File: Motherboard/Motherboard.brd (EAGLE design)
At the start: 87.5 x 150 mm, 11 parts

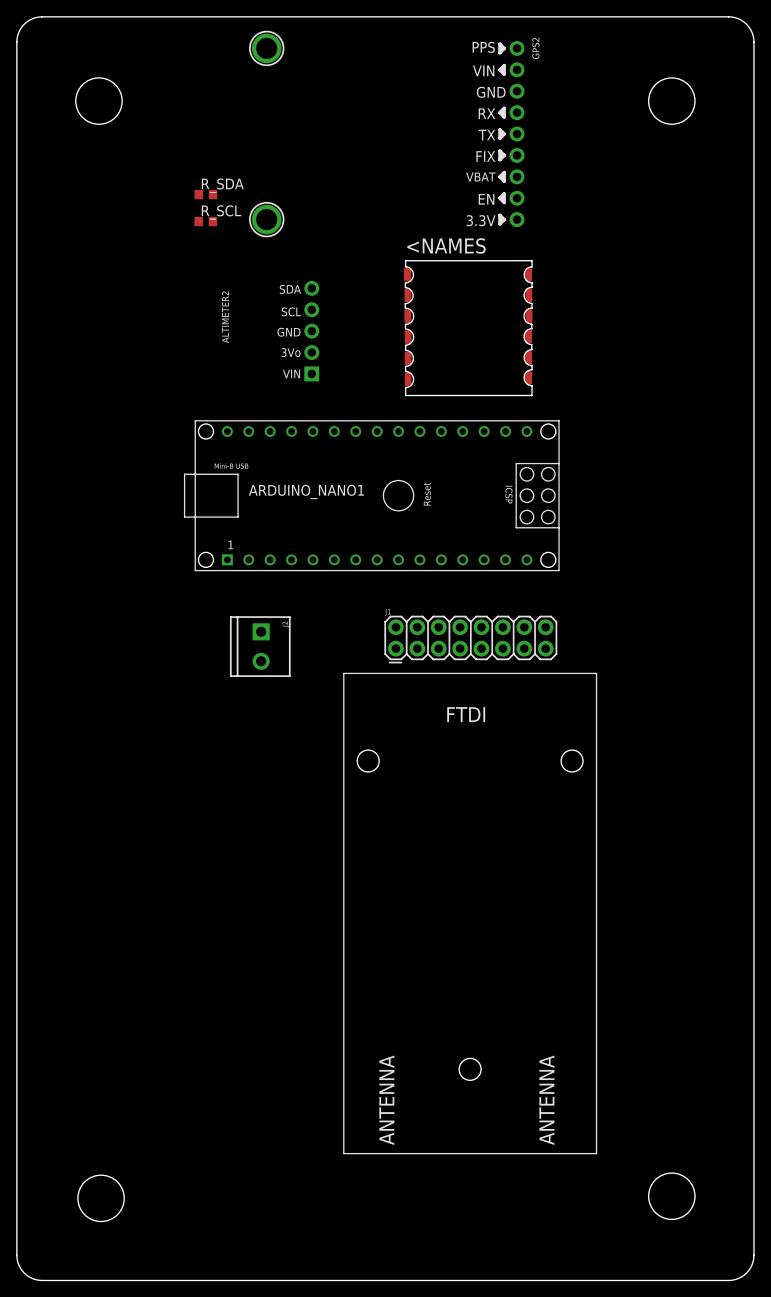
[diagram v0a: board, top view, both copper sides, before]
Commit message: refactor
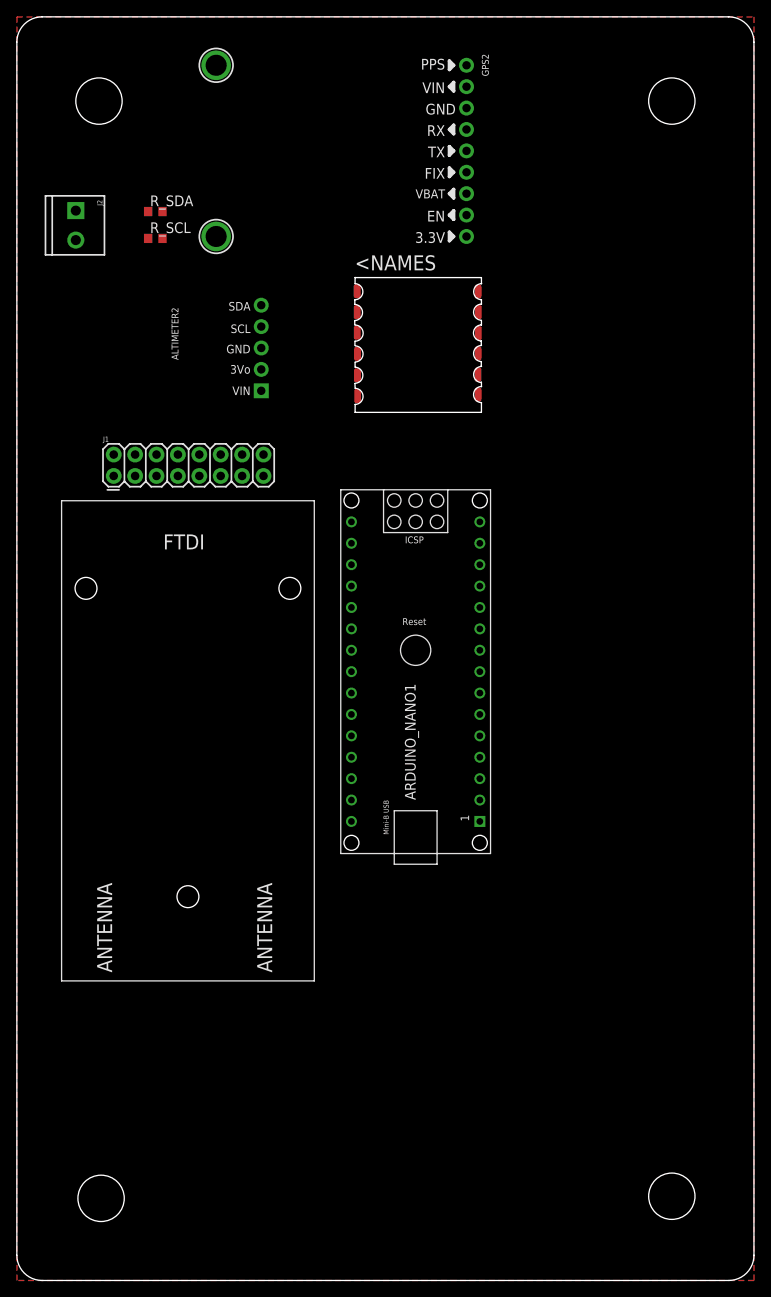
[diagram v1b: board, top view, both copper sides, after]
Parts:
- moved J2 54.6 mm to (7.00, 127.0)
- moved J1 39.3 mm to (11.5, 95.5)
- moved U$1 39.3 mm to (19.7, 64.0)
- moved ARDUINO_NANO1 18.5 mm to (47.3, 74.8), turned to 90 degrees
- moved GPS2 6.32 mm to (53.4, 134.1)
- moved IMU 6.32 mm to (37.9, 110.2)
- moved R_SCL 6.32 mm to (16.4, 123.7)
- moved U$3 6.32 mm to (23.7, 123.9)
- moved U$4 6.32 mm to (23.7, 144.2)
- moved ALTIMETER2 6.32 mm to (29.0, 110.7)
- moved R_SDA 6.32 mm to (16.4, 126.9)
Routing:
- added copper zone on layer 1, net GND
